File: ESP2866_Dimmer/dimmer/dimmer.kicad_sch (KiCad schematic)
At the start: 44 parts, among them J1 Conn_01x03_Male, J2 Screw_Terminal_01x02, J3 Conn_01x03_Male, J4 Conn_01x04_Male, J5 Screw_Terminal_01x02, J6 Screw_Terminal_01x02, J7 Screw_Terminal_01x02, K1 TIANBO-HJR-4102-L, Q1 2N3904, SW1 SW_Push, U1 LDH-45A-350, U2 B1203S-1WR3, U3 ESP-12E, U4 LTV-354T, U5 LTV-354T, U6 LTV-354T, U7 LTV-354T, U8 LTV-354T, U9 L78L05_SOT89

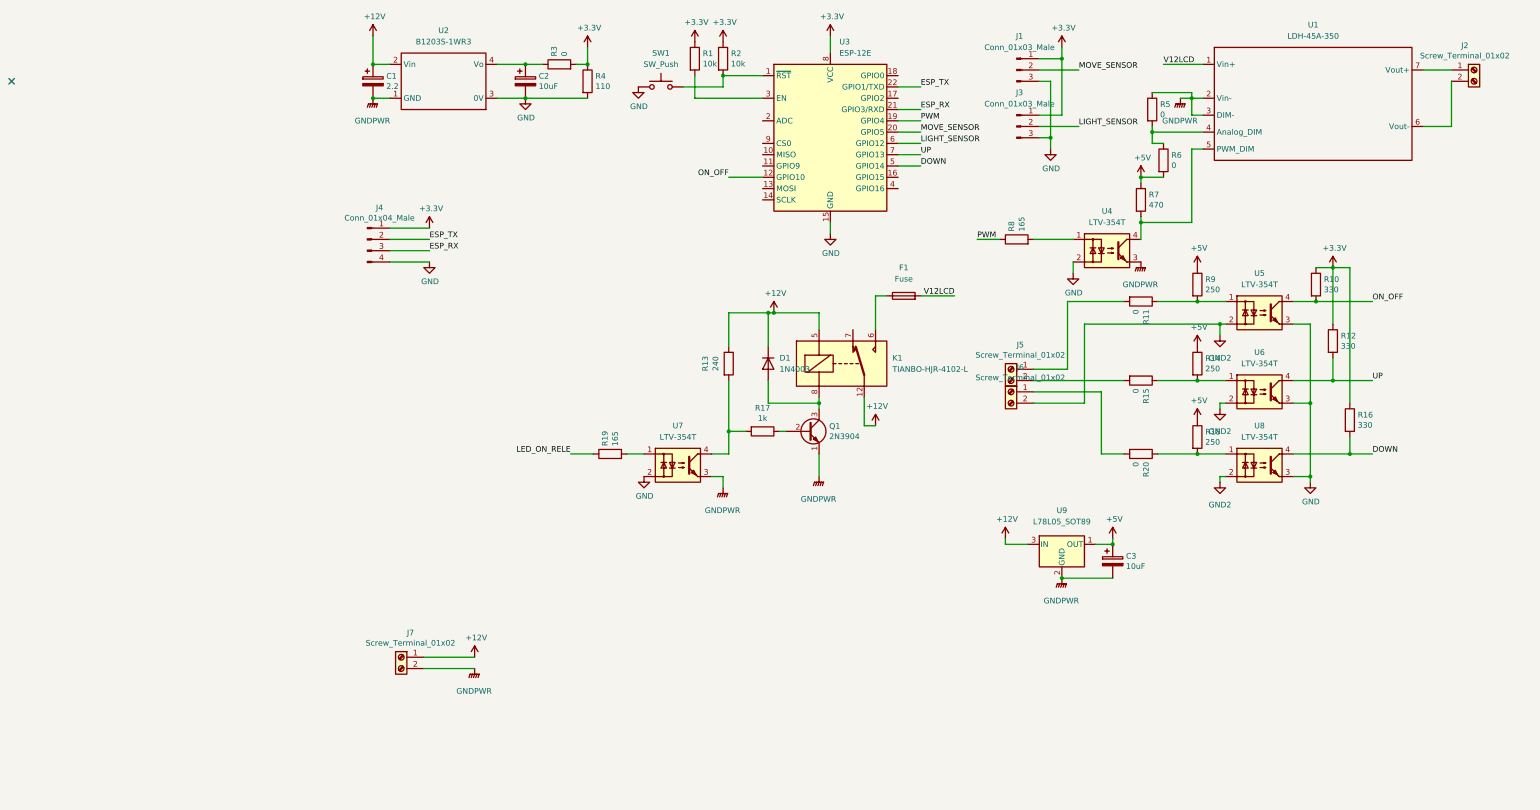
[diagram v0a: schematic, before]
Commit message: Big Update.
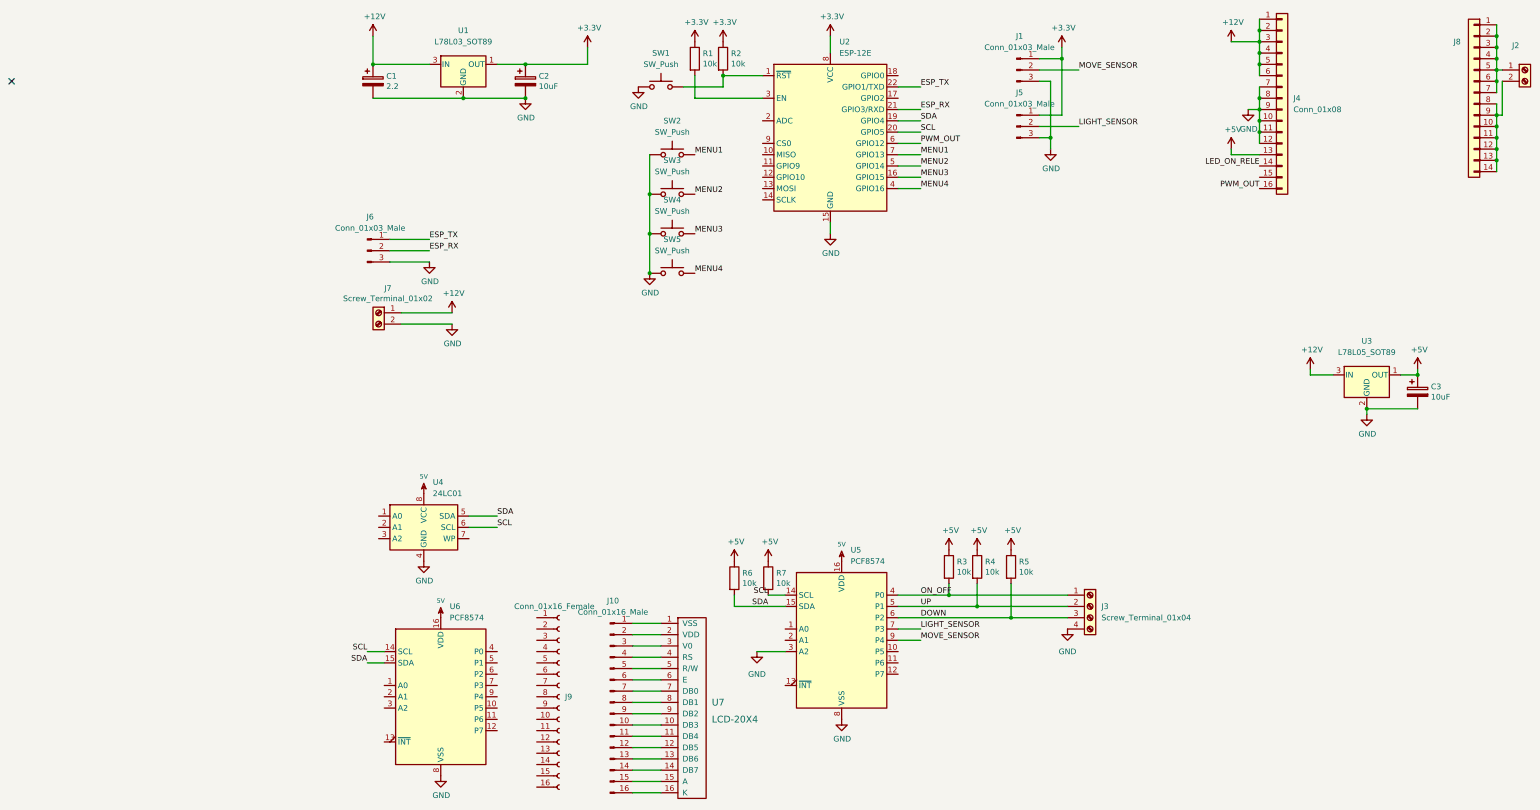
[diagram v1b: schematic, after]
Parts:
- removed D1: 1N4003, Diode_SMD:D_SMA, symbol Diode:1N4003
- removed F1: Fuse, Fuse:Fuse_2920_7451Metric_Pad2.10x5.45mm_HandSolder, symbol Device:Fuse
- removed J4: Conn_01x04_Male, Connector_Stocko:Stocko_MKS_1654-6-0-404_1x4_P2.50mm_Vertical, symbol Connector:Conn_01x04_Male
- removed J5, J6: Screw_Terminal_01x02, Connector_JST:JST_NV_B02P-NV_1x02_P5.00mm_Vertical, symbol Connector:Screw_Terminal_01x02
- removed K1: TIANBO-HJR-4102-L, Relay_THT:Relay_SPDT_HJR-4102, symbol Relay:TIANBO-HJR-4102-L
- removed Q1: 2N3904, Package_TO_SOT_THT:TO-92_Inline, symbol Transistor_BJT:2N3904
- removed R10, R12, R16: 330, Resistor_SMD:R_1206_3216Metric_Pad1.30x1.75mm_HandSolder, symbol Device:R
- removed R11, R15, R20, R3, R5: 0, Resistor_SMD:R_1206_3216Metric_Pad1.30x1.75mm_HandSolder, symbol Device:R
- removed R13: 240, Resistor_SMD:R_1206_3216Metric_Pad1.30x1.75mm_HandSolder, symbol Device:R
- removed R17: 1k, Resistor_SMD:R_1206_3216Metric_Pad1.30x1.75mm_HandSolder, symbol Device:R
- removed R19, R8: 165, Resistor_SMD:R_1206_3216Metric_Pad1.30x1.75mm_HandSolder, symbol Device:R
- removed R4: 110, Resistor_SMD:R_1206_3216Metric_Pad1.30x1.75mm_HandSolder, symbol Device:R
- removed U1: LDH-45A-350, dimmer:LDH-45A, symbol dimmer_lib:LDH-45A-350
- removed U2: B1203S-1WR3, dimmer:B1203-1WR3, symbol dimmer_lib:B1205S-1WR3
- removed U4, U5, U6, U7, U8: LTV-354T, Package_SO:SO-4_4.4x3.6mm_P2.54mm, symbol Isolator:LTV-354T
- added J10: Conn_01x16_Male, symbol Connector:Conn_01x16_Male
- added J3: Screw_Terminal_01x04, Connector_JST:JST_NV_B04P-NV_1x04_P5.00mm_Vertical, symbol Connector:Screw_Terminal_01x04
- added J4: Conn_01x08, Connector_PinSocket_1.27mm:PinSocket_1x16_P1.27mm_Vertical, symbol Connector_Generic:Conn_01x16
- added J6: Conn_01x03_Male, Connector_JST:JST_EH_B3B-EH-A_1x03_P2.50mm_Vertical, symbol Connector:Conn_01x03_Male
- added J8: Conn_01x06, Connector_PinSocket_1.27mm:PinSocket_1x14_P1.27mm_Vertical, symbol Connector_Generic:Conn_01x14
- added J9: Conn_01x16_Female, symbol Connector:Conn_01x16_Female
- added SW2, SW3, SW4, SW5: SW_Push, Button_Switch_THT:SW_PUSH_6mm, symbol Switch:SW_Push
- added U1: L78L03_SOT89, Package_TO_SOT_SMD:SOT-89-3, symbol Regulator_Linear:L78L05_SOT89
- added U4: 24LC01, Package_SO:SOIC-8_3.9x4.9mm_P1.27mm, symbol Memory_EEPROM:24LC01
- added U5, U6: PCF8574, Package_SO:SOIC-16W_7.5x10.3mm_P1.27mm, symbol Interface_Expansion:PCF8574
- added U7: LCD-20X4, symbol tinkerforge:LCD-20X4
- R3: renamed from R18; value 250 -> 10k
- R4: renamed from R14; value 250 -> 10k
- R5: renamed from R9; value 250 -> 10k
- R6: value 0 -> 10k
- R7: value 470 -> 10k
- renumbered J3 to J5, U3 to U2, U9 to U3
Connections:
- net GNDPWR is gone; now on net GND: C1.2, C3.2, J7.2 (Pin_2), U3.2 (GND)
- net +12V: now also J4.1 (Pin_1), J4.2 (Pin_2), J4.3 (Pin_3), J4.4 (Pin_4), J4.5 (Pin_5), J4.6 (Pin_6), U1.3 (IN)
- net +3V3: now also C2.1, U1.1 (OUT)
- net +5V: now also R6.1, J4.13 (Pin_13); no longer R6.2
- net DOWN: now also R5.2, J3.3 (Pin_3), U5.6 (P2); no longer U2.5 (GPIO14)
- net ESP_RX: now also J6.2 (Pin_2)
- net ESP_TX: now also J6.1 (Pin_1)
- net GND: now also J3.4 (Pin_4), J4.10 (Pin_10), J4.11 (Pin_11), J4.12 (Pin_12), J4.7 (Pin_7), J4.8 (Pin_8), J4.9 (Pin_9), J6.3 (Pin_3), SW2.1, SW3.1, SW4.1, SW5.1, U1.2 (GND), U4.4 (GND), U5.3 (A2), U5.8 (VSS), U6.8 (VSS)
- net LED_ON_RELE: now also J4.14 (Pin_14)
- net LIGHT_SENSOR: now also U5.7 (P3); no longer U2.6 (GPIO12)
- net MOVE_SENSOR: now also U5.9 (P4); no longer U2.20 (GPIO5)
- net ON_OFF: now also R3.2, J3.1 (Pin_1), U5.4 (P0); no longer U2.12 (GPIO10)
- net UP: now also R4.2, J3.2 (Pin_2), U5.5 (P1); no longer U2.7 (GPIO13)
- net MENU3: now reaches U2.16 (GPIO15)
- net MENU3: now also SW4.2
- net MENU4: now reaches U2.4 (GPIO16)
- net MENU4: now also SW5.2
- net at J2.1 (Pin_1): now also J8.1 (Pin_1), J8.2 (Pin_2), J8.3 (Pin_3), J8.4 (Pin_4), J8.5 (Pin_5), J8.6 (Pin_6), J8.7 (Pin_7)
- net at J2.2 (Pin_2): now also J8.10 (Pin_10), J8.11 (Pin_11), J8.12 (Pin_12), J8.13 (Pin_13), J8.14 (Pin_14), J8.8 (Pin_8), J8.9 (Pin_9)
- net SCL: now reaches R7.2
- net SCL: now also U2.20 (GPIO5), U4.6 (SCL), U5.14 (SCL), U6.14 (SCL)
- net PWM renamed SDA
- net SDA: now also R6.2, U4.5 (SDA), U5.15 (SDA), U6.15 (SDA)
- new net: J10.1 (Pin_1), U7.1 (VSS)
- new net: J10.10 (Pin_10), U7.10 (DB3)
- new net: J10.11 (Pin_11), U7.11 (DB4)
- new net: J10.12 (Pin_12), U7.12 (DB5)
- new net: J10.13 (Pin_13), U7.13 (DB6)
- new net: J10.14 (Pin_14), U7.14 (DB7)
- new net: J10.15 (Pin_15), U7.15 (A)
- new net: J10.16 (Pin_16), U7.16 (K)
- new net: J10.2 (Pin_2), U7.2 (VDD)
- new net: J10.3 (Pin_3), U7.3 (V0)
- new net: J10.4 (Pin_4), U7.4 (RS)
- new net: J10.5 (Pin_5), U7.5 (R/W)
- new net: J10.6 (Pin_6), U7.6 (E)
- new net: J10.7 (Pin_7), U7.7 (DB0)
- new net: J10.8 (Pin_8), U7.8 (DB1)
- new net: J10.9 (Pin_9), U7.9 (DB2)
- new net 5V: U4.8 (VCC), U5.16 (VDD), U6.16 (VDD)
- new net MENU1: SW2.2, U2.7 (GPIO13)
- new net MENU2: SW3.2, U2.5 (GPIO14)
- new net PWM_OUT: J4.16 (Pin_16), U2.6 (GPIO12)
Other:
- moved on the sheet: C3, J2, J7, R3, R4, R5, U3
